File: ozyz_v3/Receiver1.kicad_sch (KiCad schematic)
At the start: 12 parts, among them J5 AudioJack4, Q8 2N7002

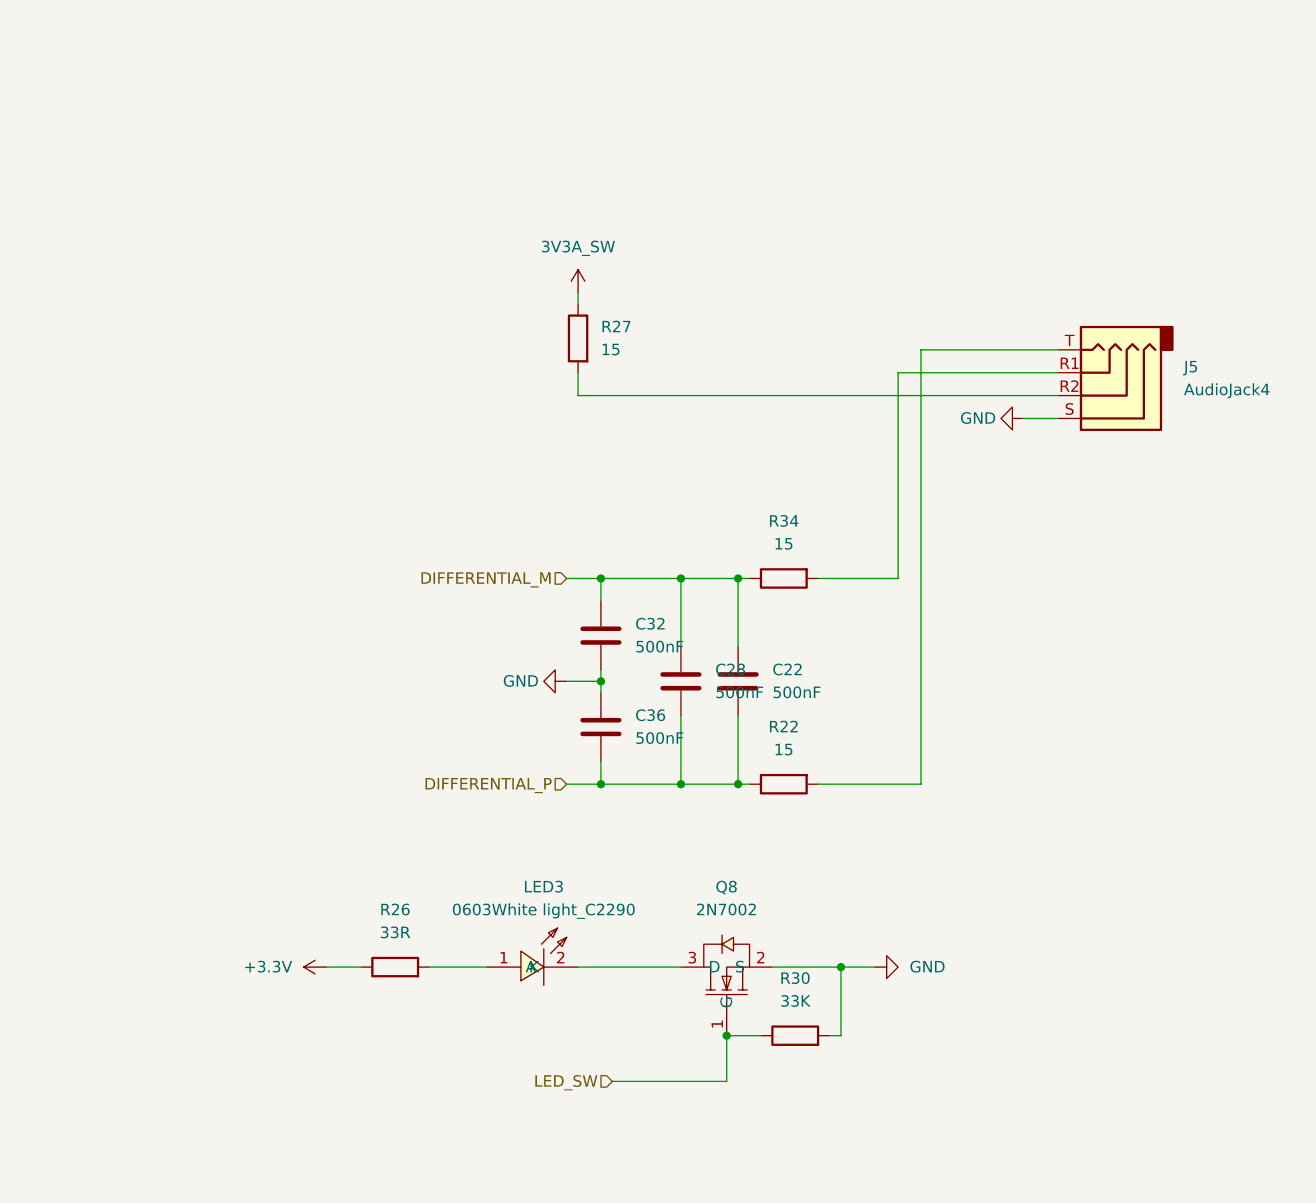
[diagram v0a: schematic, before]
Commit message: OZYS ready for layout
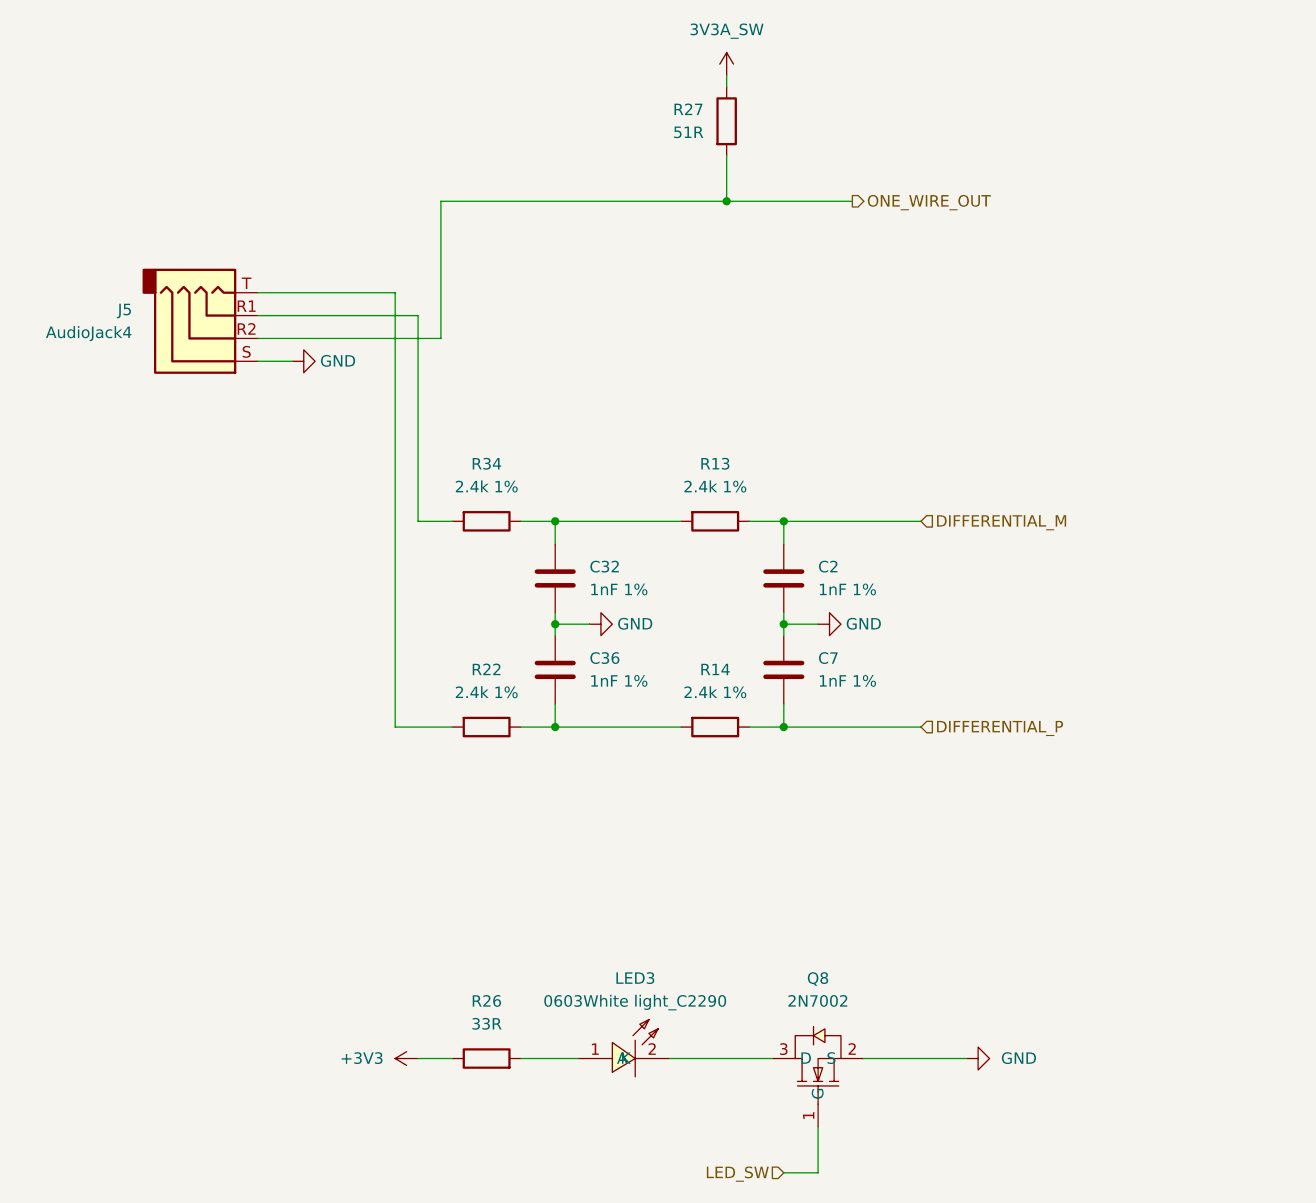
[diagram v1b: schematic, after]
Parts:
- removed C22, C28: 500nF, symbol Device:C
- removed R30: 33K, Resistor_SMD:R_0402_1005Metric, symbol Device:R
- added C2, C7: 1nF 1%, Capacitor_SMD:C_0603_1608Metric_Pad1.08x0.95mm_HandSolder, symbol Device:C
- added R13, R14: 2.4k 1%, Capacitor_SMD:C_0603_1608Metric_Pad1.08x0.95mm_HandSolder, symbol Device:R
- C32, C36: value 500nF -> 1nF 1%; footprint (none) -> Capacitor_SMD:C_0603_1608Metric_Pad1.08x0.95mm_HandSolder
- J5: footprint Rocketry_Easyeda:AUDIO-TH_PJ-320A-4P-DIP -> Rocketry_Manual:AUDIO-TH_PJ-320A-4P-DIP
- R22, R34: value 15 -> 2.4k 1%; footprint (none) -> Capacitor_SMD:C_0603_1608Metric_Pad1.08x0.95mm_HandSolder
- R27: value 15 -> 51R; footprint (none) -> Resistor_SMD:R_0402_1005Metric
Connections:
- net DIFFERENTIAL_M: now also C2.1, R13.1; no longer C32.1, R34.1
- net DIFFERENTIAL_P: now also C7.2, R14.1; no longer C36.2, R22.1
- net GND: now also C2.2, C7.1
- net ONE_WIRE_OUT: now reaches J5.R2, R27.2
- net +3.3V renamed +3V3
- new net: C36.2, R14.2, R22.1
- new net: C32.1, R13.2, R34.1
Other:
- moved on the sheet: C32, C36, J5, LED3, Q8, R22, R26, R27, R34
